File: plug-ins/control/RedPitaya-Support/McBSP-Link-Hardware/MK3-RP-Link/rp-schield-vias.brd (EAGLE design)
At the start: 59 x 55.3 mm, 21 parts, among them U1 SN65MLVD202A, U2 SN65MLVD202A, U3 SN65MLVD202A

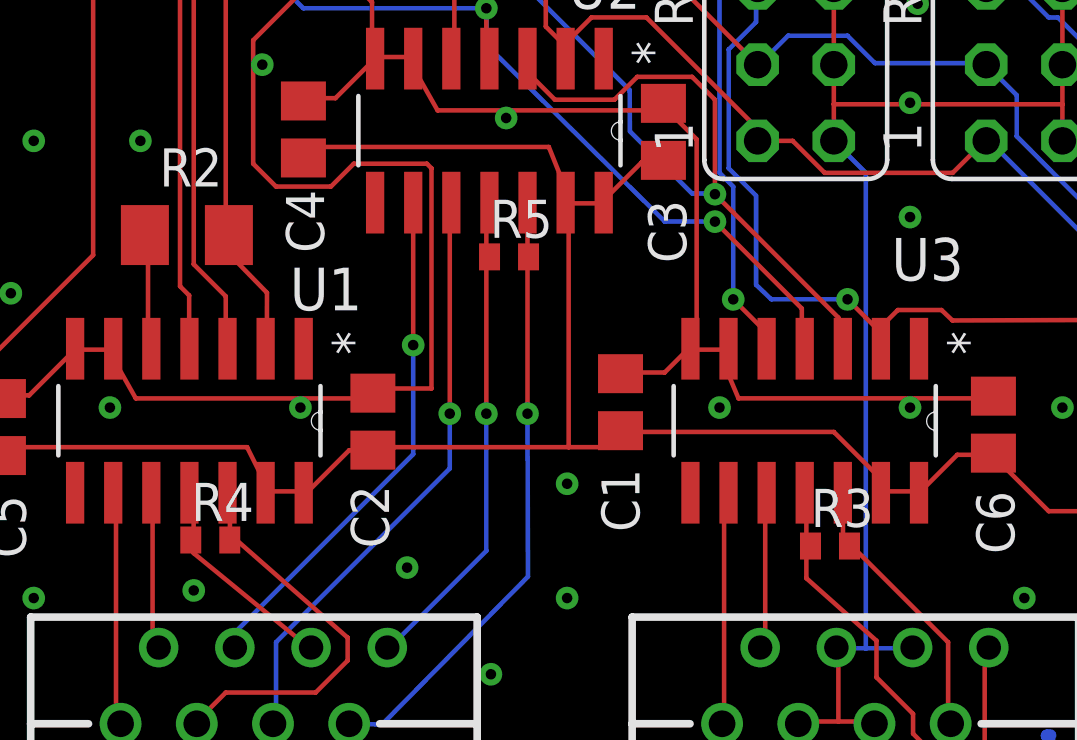
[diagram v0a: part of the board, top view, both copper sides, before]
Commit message: minor updates, cleanups
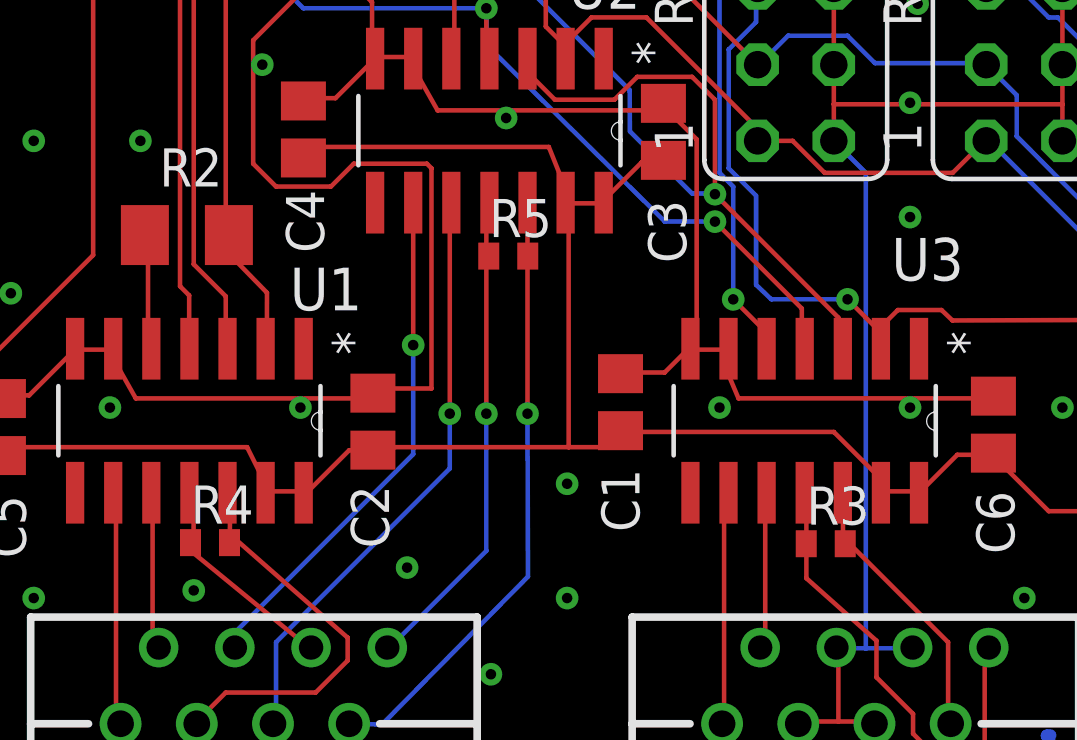
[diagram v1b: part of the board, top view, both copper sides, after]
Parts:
- moved R3 0.16 mm to (41.6, 24.7)
- moved R4 0.09 mm to (21.1, 24.7)
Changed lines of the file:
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@@
 <drawing>
 <settings>
-<setting alwaysvectorfont="no"/>
+<setting alwaysvectorfont="yes"/>
 <setting verticaltext="up"/>
 </settings>
@@
 <attribute name="VALUE" x="45.339" y="36.83" size="1.27" layer="27" ratio="10" rot="R90"/>
 </element>
-<element name="R3" library="resistor" library_urn="urn:adsk.eagle:library:348" package="R0402" package3d_urn="urn:adsk.eagle:package:26058/1" value="100R" x="41.7823125" y="24.594221875"/>
-<element name="R4" library="resistor" library_urn="urn:adsk.eagle:library:348" package="R0402" package3d_urn="urn:adsk.eagle:package:26058/1" value="100R" x="21.125246875" y="24.7952"/>
-<element name="R5" library="resistor" library_urn="urn:adsk.eagle:library:348" package="R0402" package3d_urn="urn:adsk.eagle:package:26058/1" value="100R" x="31.083778125" y="34.232609375"/>
+<element name="R3" library="resistor" library_urn="urn:adsk.eagle:library:348" package="R0402" package3d_urn="urn:adsk.eagle:package:26058/1" value="100R" x="41.6412375" y="24.671178125"/>
+<element name="R4" library="resistor" library_urn="urn:adsk.eagle:library:348" package="R0402" package3d_urn="urn:adsk.eagle:package:26058/1" value="100R" x="21.1160125" y="24.7075625"/>
+<element name="R5" library="resistor" library_urn="urn:adsk.eagle:library:348" package="R0402" package3d_urn="urn:adsk.eagle:package:26058/1" value="100R" x="31.058128125" y="34.258259375"/>
 </elements>
 <signals>
@@
 <wire x1="45.72" y1="18.796" x2="45.805" y2="18.67" width="0.1524" layer="1"/>
 <contactref element="R3" pad="2"/>
-<wire x1="42.4323125" y1="24.594221875" x2="42.2148" y2="24.892" width="0" layer="19" extent="1-1"/>
+<wire x1="42.2912375" y1="24.671178125" x2="42.2148" y2="24.892" width="0" layer="19" extent="1-1"/>
 </signal>
 <signal name="MOSI-">
@@
 <wire x1="46.9392" y1="21.082" x2="47.075" y2="21.21" width="0.1524" layer="1"/>
 <contactref element="R3" pad="1"/>
-<wire x1="40.9956" y1="23.5204" x2="41.1323125" y2="24.594221875" width="0" layer="19" extent="1-1"/>
+<wire x1="40.9956" y1="23.5204" x2="40.9912375" y2="24.671178125" width="0" layer="19" extent="1-1"/>
 </signal>
 <signal name="CS+RET-FSR">
@@
 <wire x1="20.7264" y1="18.796" x2="20.675" y2="18.67" width="0.1524" layer="1"/>
 <contactref element="R4" pad="2"/>
-<wire x1="21.776109375" y1="24.989340625" x2="21.775246875" y2="24.7952" width="0" layer="19" extent="1-1"/>
+<wire x1="21.776109375" y1="24.989340625" x2="21.7660125" y2="24.7075625" width="0" layer="19" extent="1-1"/>
 </signal>
 <signal name="CS-FSX">
@@
 <wire x1="24.384" y1="21.2344" x2="24.485" y2="21.21" width="0.1524" layer="1"/>
 <contactref element="R4" pad="1"/>
-<wire x1="20.475246875" y1="24.7952" x2="20.56545625" y2="24.36075625" width="0" layer="19" extent="1-1"/>
+<wire x1="20.4660125" y1="24.7075625" x2="20.56545625" y2="24.36075625" width="0" layer="19" extent="1-1"/>
 </signal>
 <signal name="CLK+-CLKX">
@@
 <via x="31.6992" y="29.0068" extent="1-16" drill="0.35"/>
 <contactref element="R5" pad="2"/>
-<wire x1="31.6992" y1="36.0172" x2="31.733778125" y2="34.232609375" width="0" layer="19" extent="1-1"/>
+<wire x1="31.6992" y1="36.0172" x2="31.708128125" y2="34.258259375" width="0" layer="19" extent="1-1"/>
 </signal>
 <signal name="CLK-RET-CLKR">
@@
 <via x="30.3276" y="29.0068" extent="1-16" drill="0.35"/>
 <contactref element="R5" pad="1"/>
-<wire x1="30.3276" y1="36.0172" x2="30.433778125" y2="34.232609375" width="0" layer="19" extent="1-1"/>
+<wire x1="30.3276" y1="36.0172" x2="30.408128125" y2="34.258259375" width="0" layer="19" extent="1-1"/>
 </signal>
 <signal name="~RE">
